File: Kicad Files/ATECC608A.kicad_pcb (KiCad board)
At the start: 2 copper layers, 26.7 x 22.8 mm, 21 parts, among them J1 Conn_01x04, U1 ATECC608A-SSHDA

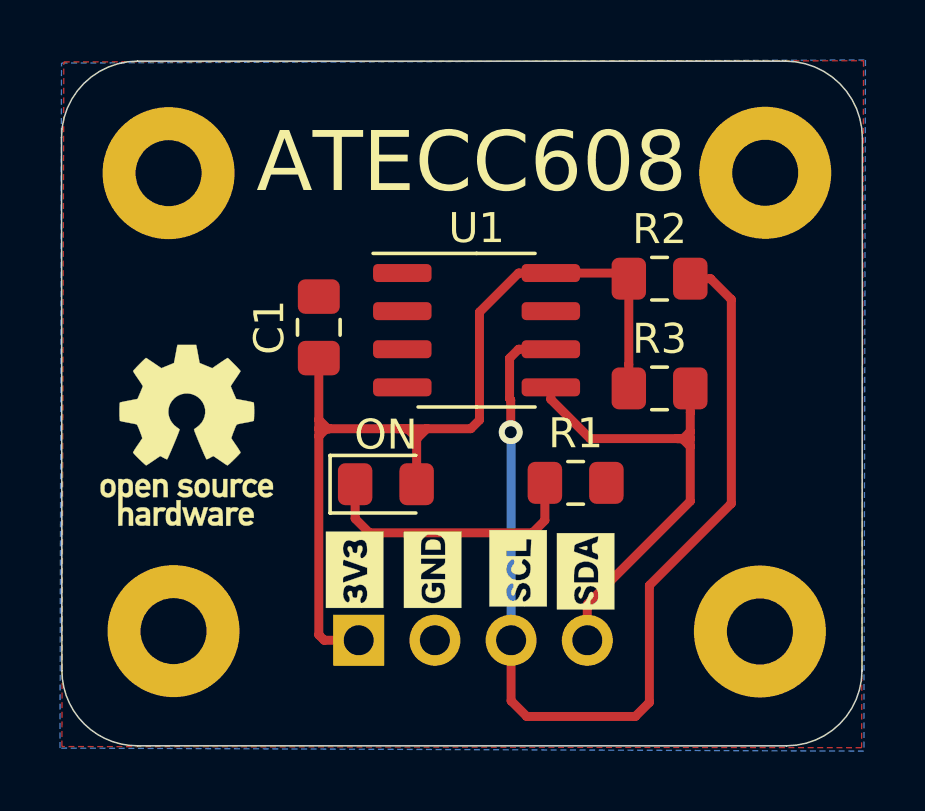
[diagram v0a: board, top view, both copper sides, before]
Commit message: logos
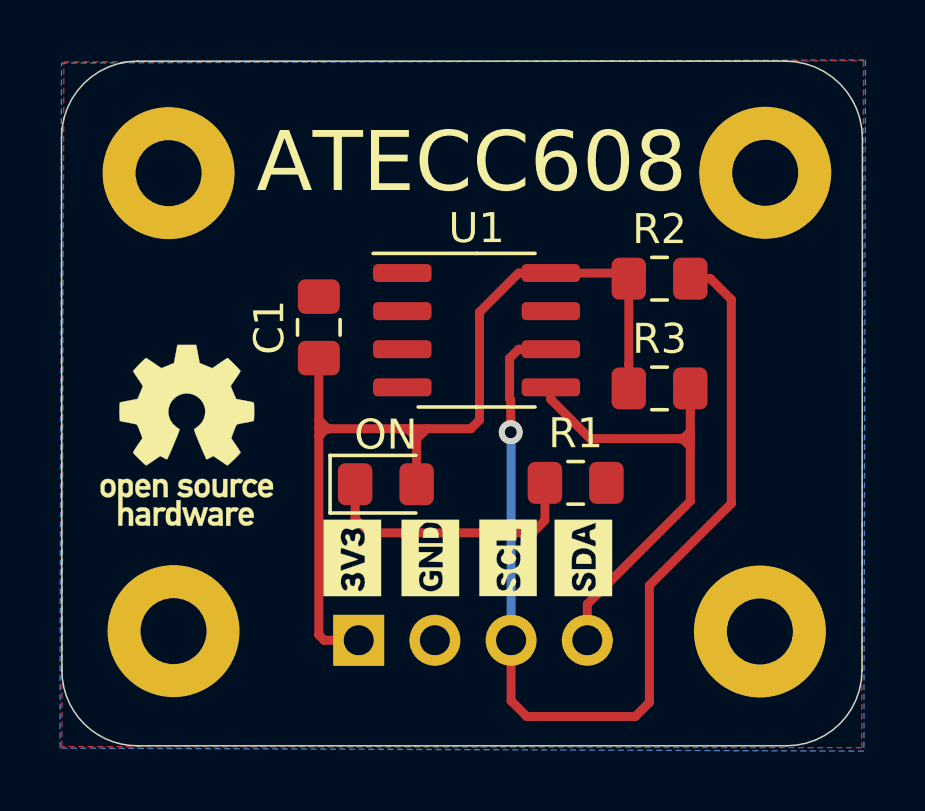
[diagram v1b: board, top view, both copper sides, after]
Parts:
- moved G*** 0.48 mm to (166.0, 47.1)
- moved G*** 0.45 mm to (168.5, 47.1)
- moved G*** 0.40 mm to (163.4, 47.1)
- moved G*** 0.40 mm to (160.8, 47.1)
- moved G*** 0.14 mm to (163.7, 47.0)
- moved G*** 0.10 mm to (161.0, 47.0)
- moved G*** 0.08 mm to (166.2, 47.0)
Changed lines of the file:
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@@
-(kicad_pcb (version 20171130) (host pcbnew "(5.1.4-0-10_14)")
+(kicad_pcb (version 20171130) (host pcbnew "(5.1.4)-1")
   (general
     (thickness 1.6)
@@
     (35 F.Paste user)
     (36 B.SilkS user)
-    (37 F.SilkS user hide)
+    (37 F.SilkS user)
     (38 B.Mask user)
     (39 F.Mask user)
@@
     (43 Eco2.User user)
     (44 Edge.Cuts user)
-    (45 Margin user)
+    (45 Margin user hide)
     (46 B.CrtYd user)
     (47 F.CrtYd user)
@@
   )
   (module Aesthetics:SCL (layer B.Cu)
-    (at 166.15 47.125 270)
+    (at 166.15 47.05 270)
     (fp_text reference G*** (at 0 0 90) (layer B.SilkS) hide
       (effects (font (size 1.524 1.524) (thickness 0.3)) (justify mirror))
@@
   )
   (module Aesthetics:GND (layer B.Cu)
-    (at 163.575 47.1 270)
+    (at 163.703 47.05 270)
     (fp_text reference G*** (at 0 0 90) (layer B.SilkS) hide
       (effects (font (size 1.524 1.524) (thickness 0.3)) (justify mirror))
@@
   )
   (module Aesthetics:3v3 (layer B.Cu)
-    (at 161 47.15 270)
+    (at 161 47.05 270)
     (fp_text reference G*** (at 0 0 90) (layer B.SilkS) hide
       (effects (font (size 1.524 1.524) (thickness 0.3)) (justify mirror))
@@
   )
   (module GND (layer F.Cu)
-    (at 163.5 47.45 90)
+    (at 163.4238 47.0555 90)
     (fp_text reference G*** (at 0 0 90) (layer F.SilkS) hide
       (effects (font (size 1.524 1.524) (thickness 0.3)))
@@
   )
   (module 3v3 (layer F.Cu)
-    (at 160.9 47.45 90)
+    (at 160.8238 47.0555 90)
     (fp_text reference G*** (at 0 0 90) (layer F.SilkS) hide
       (effects (font (size 1.524 1.524) (thickness 0.3)))
@@
   )
   (module SCL (layer F.Cu)
-    (at 166.35 47.4 90)
+    (at 166.0144 47.0535 90)
     (fp_text reference G*** (at 0 0 90) (layer F.SilkS) hide
       (effects (font (size 1.524 1.524) (thickness 0.3)))
@@
   )
   (module SDA (layer F.Cu)
-    (at 168.6 47.5 90)
+    (at 168.5238 47.0555 90)
     (fp_text reference G*** (at 0 0 90) (layer F.SilkS) hide
       (effects (font (size 1.524 1.524) (thickness 0.3)))
@@
     (connect_pads (clearance 0.508))
     (min_thickness 0.254)
-    (fill (arc_segments 32) (thermal_gap 0.508) (thermal_bridge_width 0.508))
+    (fill yes (arc_segments 32) (thermal_gap 0.508) (thermal_bridge_width 0.508))
     (polygon
       (pts
@@
     (connect_pads (clearance 0.508))
     (min_thickness 0.254)
-    (fill (arc_segments 32) (thermal_gap 0.508) (thermal_bridge_width 0.508))
+    (fill yes (arc_segments 32) (thermal_gap 0.508) (thermal_bridge_width 0.508))
     (polygon
       (pts
